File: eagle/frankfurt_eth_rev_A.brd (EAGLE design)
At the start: 72.2 x 65.5 mm, 62 parts, among them IC1 PIC18F26K80, IC2 ENC28J60-SO, IC3 SN65HVD232, IC4 LM2575S, IC5 11AA02E48, IC6 MCP23A256, IC7 AT45DB041D, J2 A00-108-220-450, Q1 10 MHz, Q2 25 MHz

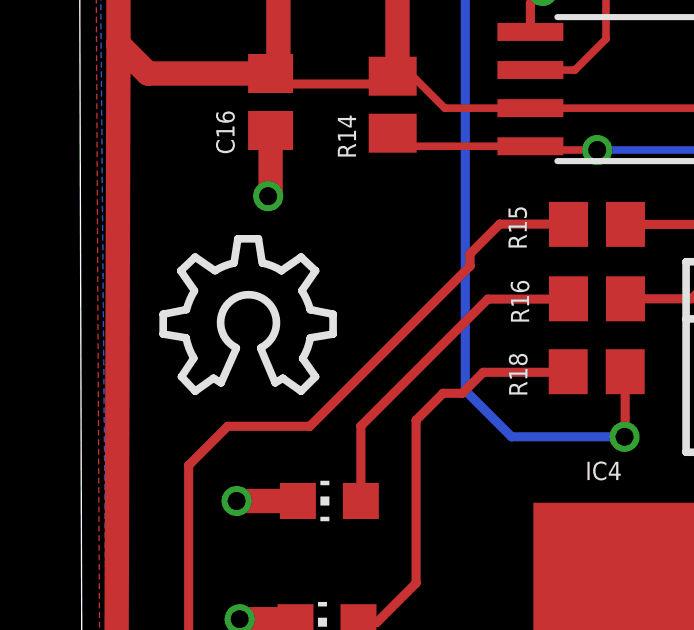
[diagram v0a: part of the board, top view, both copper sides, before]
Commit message: Edit
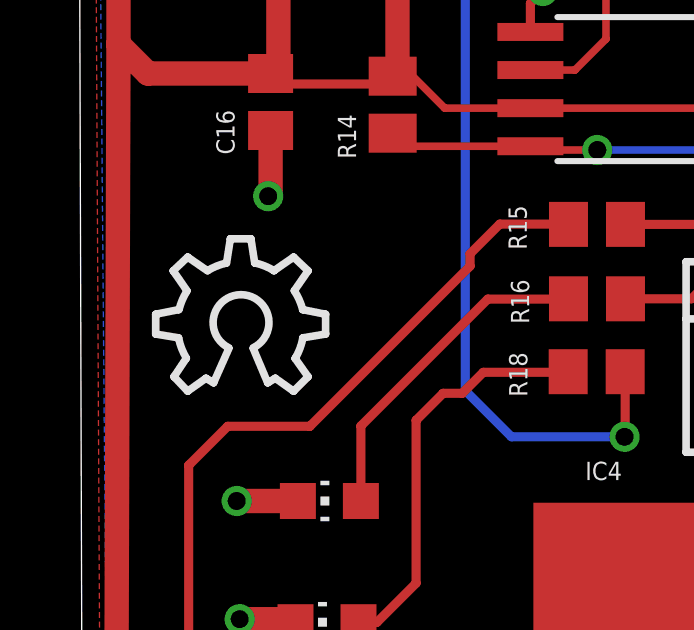
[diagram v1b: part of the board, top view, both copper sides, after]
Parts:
- moved U$2 0.25 mm to (2.44, 16.4)
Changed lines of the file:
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@@
 </element>
 <element name="U$1" library="seed_Logo" package="ROHS_SILK" value="" x="63.97" y="60.28"/>
-<element name="U$2" library="seed_Logo" package="OSHW_10X200_NOTEXT" value="" x="2.69" y="16.43"/>
+<element name="U$2" library="seed_Logo" package="OSHW_10X200_NOTEXT" value="" x="2.44" y="16.43"/>
 </elements>
 <signals>
